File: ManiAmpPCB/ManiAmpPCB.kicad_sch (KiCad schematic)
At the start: 76 parts, among them J1 Screw_Terminal_01x02, J2 Screw_Terminal_01x02, J3 Screw_Terminal_01x02, J4 Screw_Terminal_01x02, U1 ADAU1701, U2 TPA3116D2DAD, U3 TPA3116D2DAD

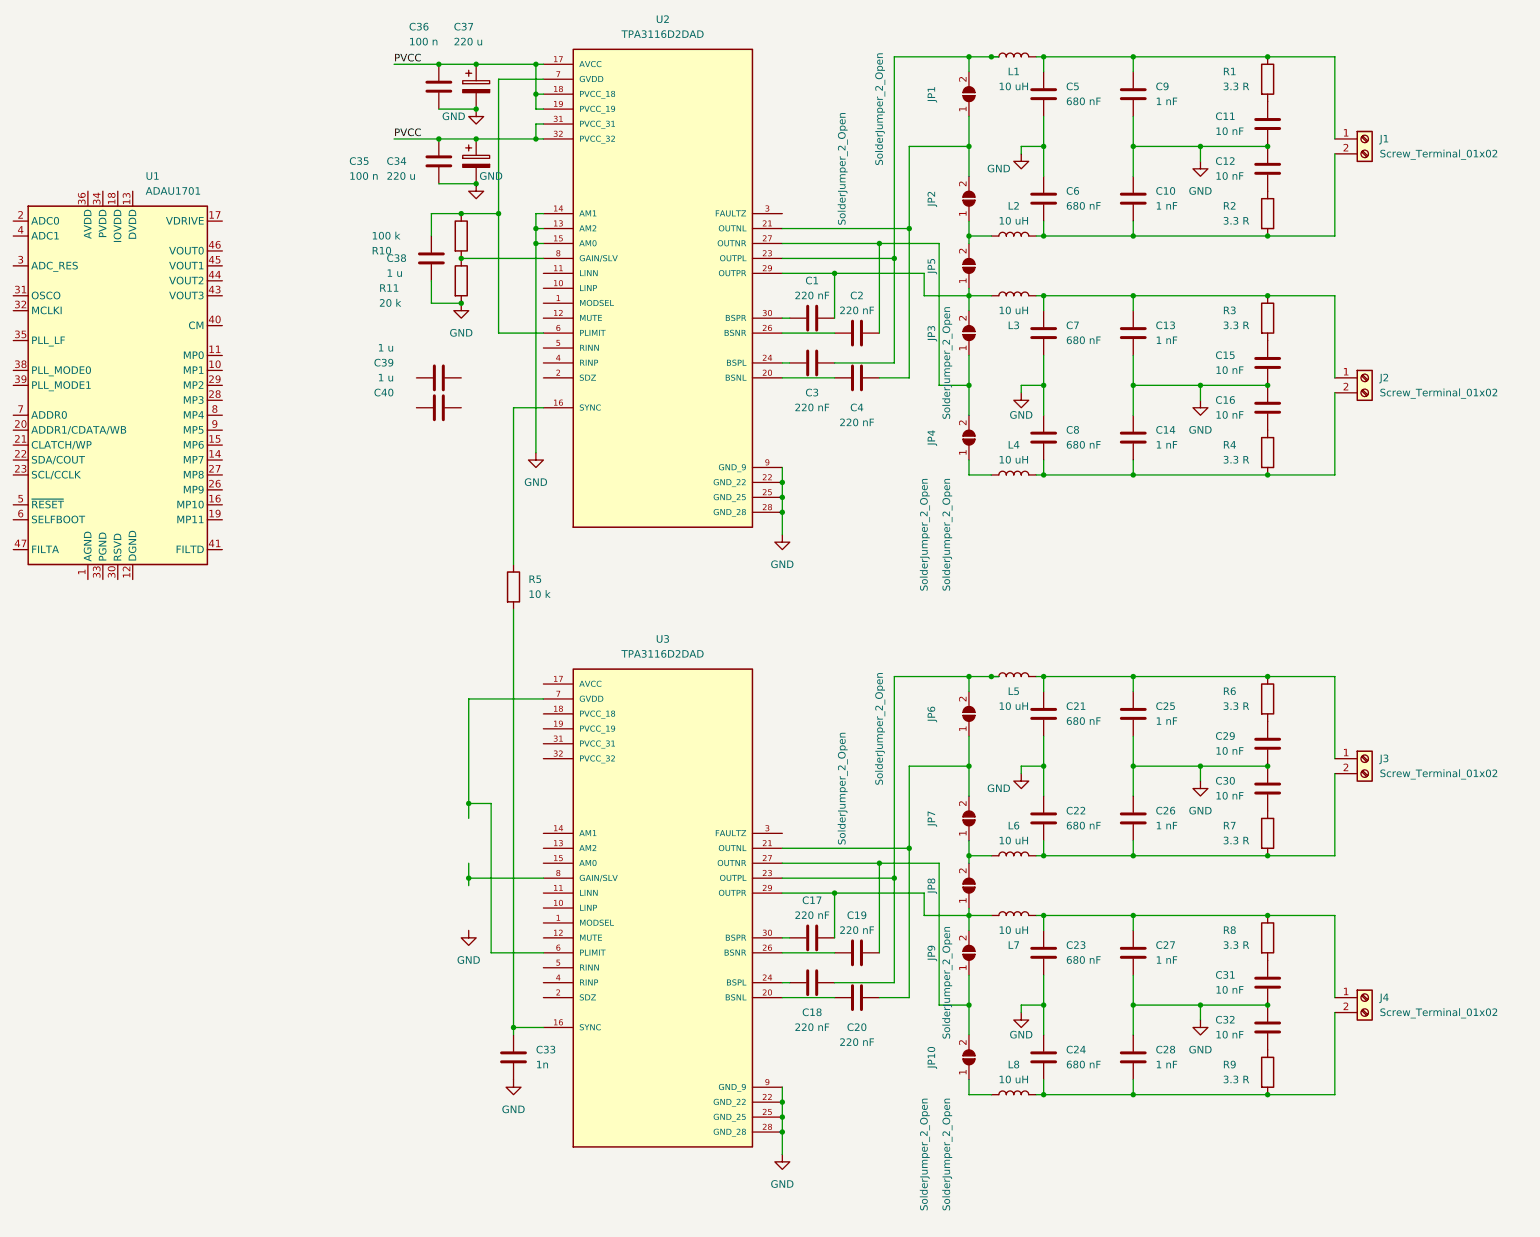
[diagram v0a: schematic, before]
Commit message: DSP schematics WiP
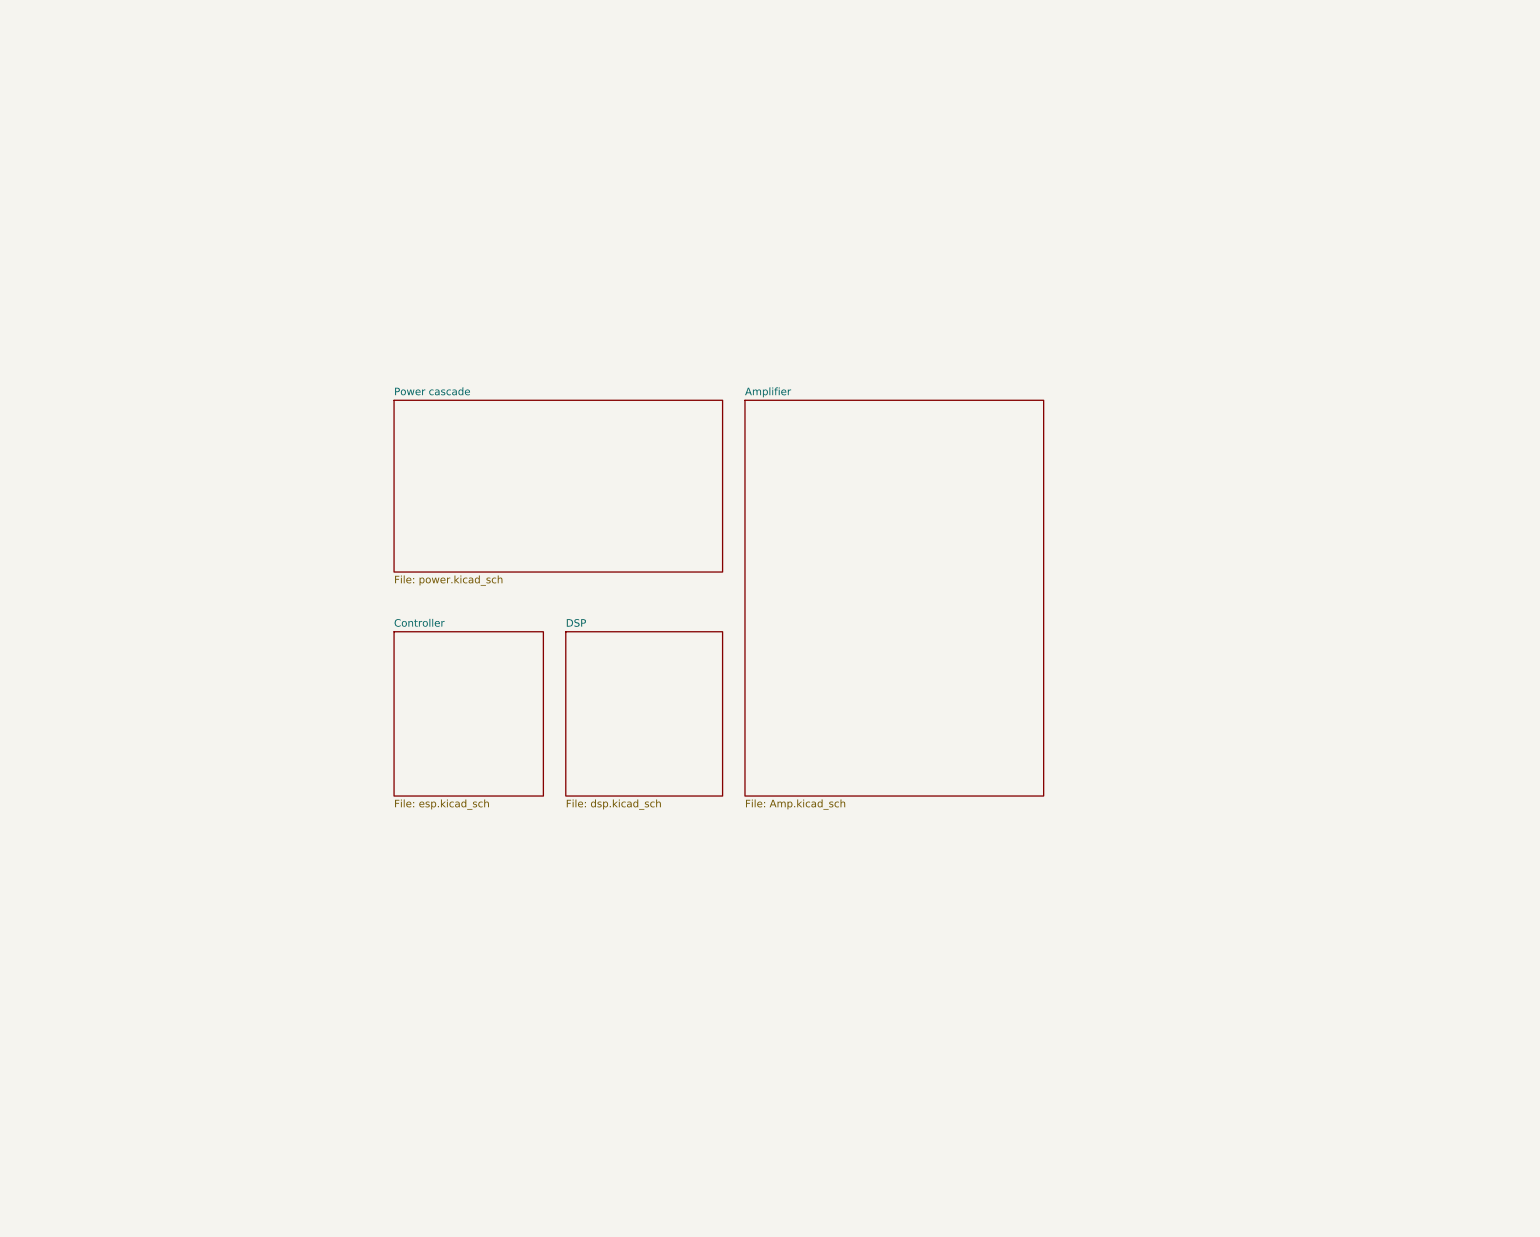
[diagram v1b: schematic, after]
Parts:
- removed C1, C17, C18, C19, C2, C20, C3, C4: 220 nF, symbol Device:C
- removed C10, C13, C14, C25, C26, C27, C28, C9: 1 nF, symbol Device:C
- removed C11, C12, C15, C16, C29, C30, C31, C32: 10 nF, symbol Device:C
- removed C21, C22, C23, C24, C5, C6, C7, C8: 680 nF, symbol Device:C
- removed C33: 1n, symbol Device:C
- removed C34, C37: 220 u, symbol Device:C_Polarized
- removed C35, C36: 100 n, symbol Device:C
- removed C38, C39, C40: 1 u, symbol Device:C
- removed J1, J2, J3, J4: Screw_Terminal_01x02, symbol Connector:Screw_Terminal_01x02
- removed JP1, JP10, JP2, JP3, JP4, JP5, JP6, JP7, JP8, JP9: SolderJumper_2_Open, symbol Jumper:SolderJumper_2_Open
- removed L1, L2, L3, L4, L5, L6, L7, L8: 10 uH, symbol Device:L
- removed R1, R2, R3, R4, R6, R7, R8, R9: 3.3 R, symbol Device:R
- removed R10: 100 k, symbol Device:R
- removed R11: 20 k, symbol Device:R
- removed R5: 10 k, symbol Device:R
- removed U1: ADAU1701, Package_QFP:LQFP-48_7x7mm_P0.5mm, symbol DSP_AnalogDevices:ADAU1701
- removed U2, U3: TPA3116D2DAD, TPA3116D2DAD:SOP65P810X115-32N, symbol Manifold:TPA3116D2DAD
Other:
- added sheet Amplifier (Amp.kicad_sch)
- added sheet Controller (esp.kicad_sch)
- added sheet DSP (dsp.kicad_sch)
- added sheet Power cascade (power.kicad_sch)
